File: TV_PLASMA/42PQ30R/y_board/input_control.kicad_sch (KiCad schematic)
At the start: 1 part, among them P101 Conn_02x15_Counter_Clockwise

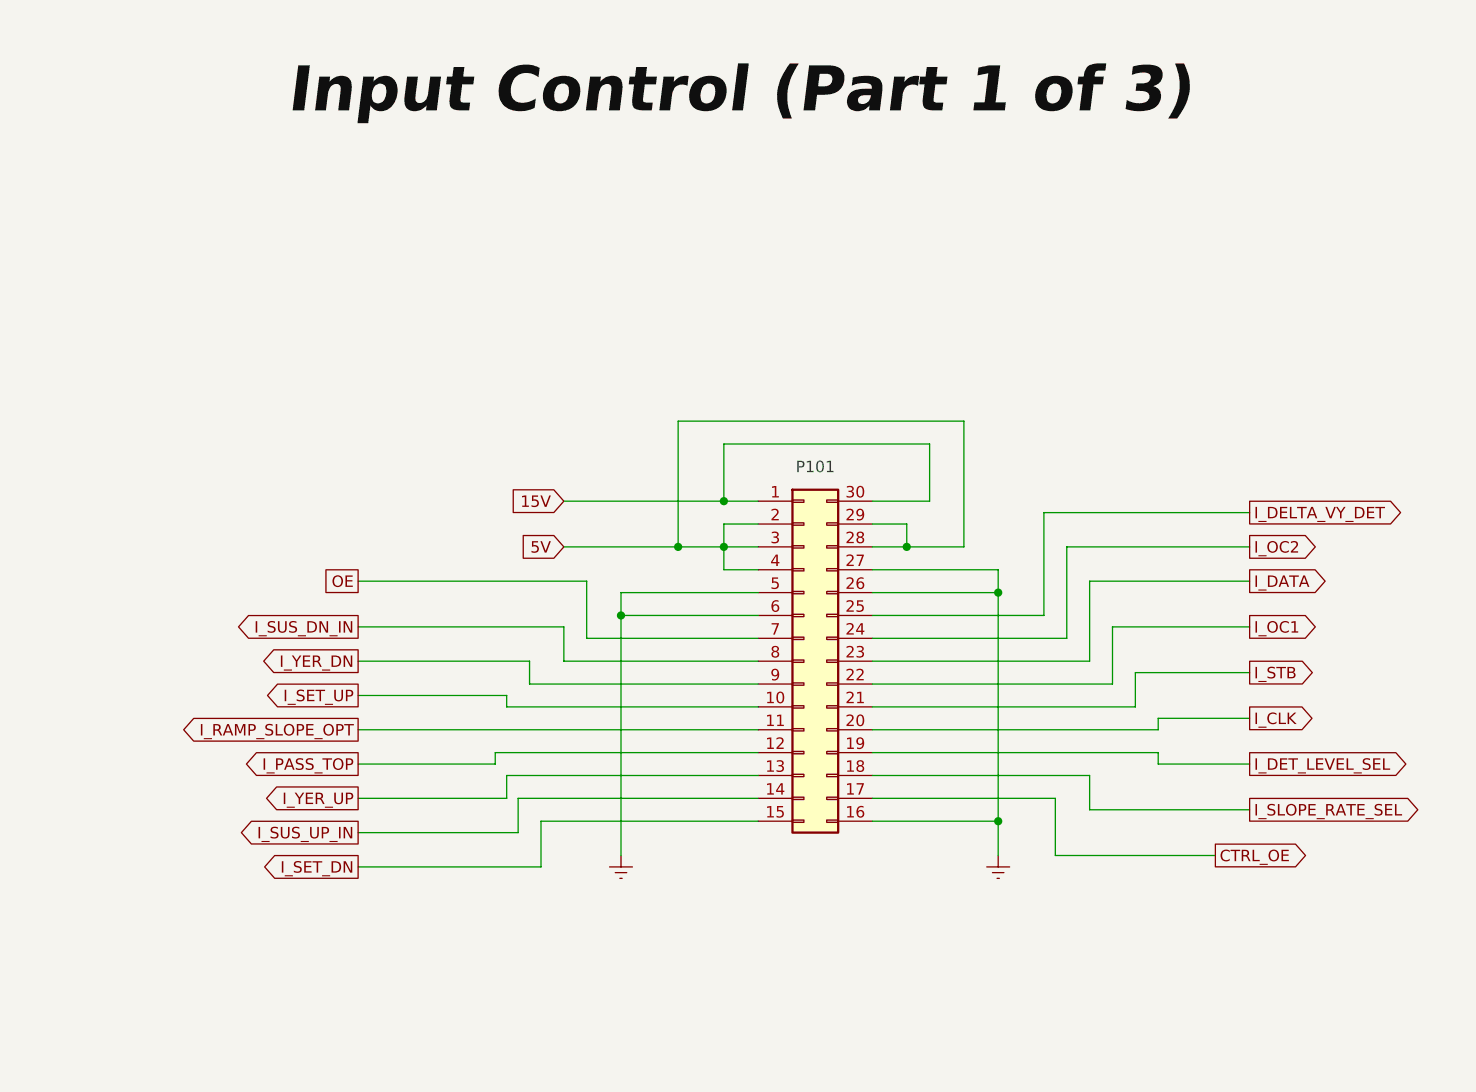
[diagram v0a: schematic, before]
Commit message: Finishing Y BOARD reverse engineering. Todo: Add reverse conduction and resistence to all output/input pins and refactor Z BOARD DRC
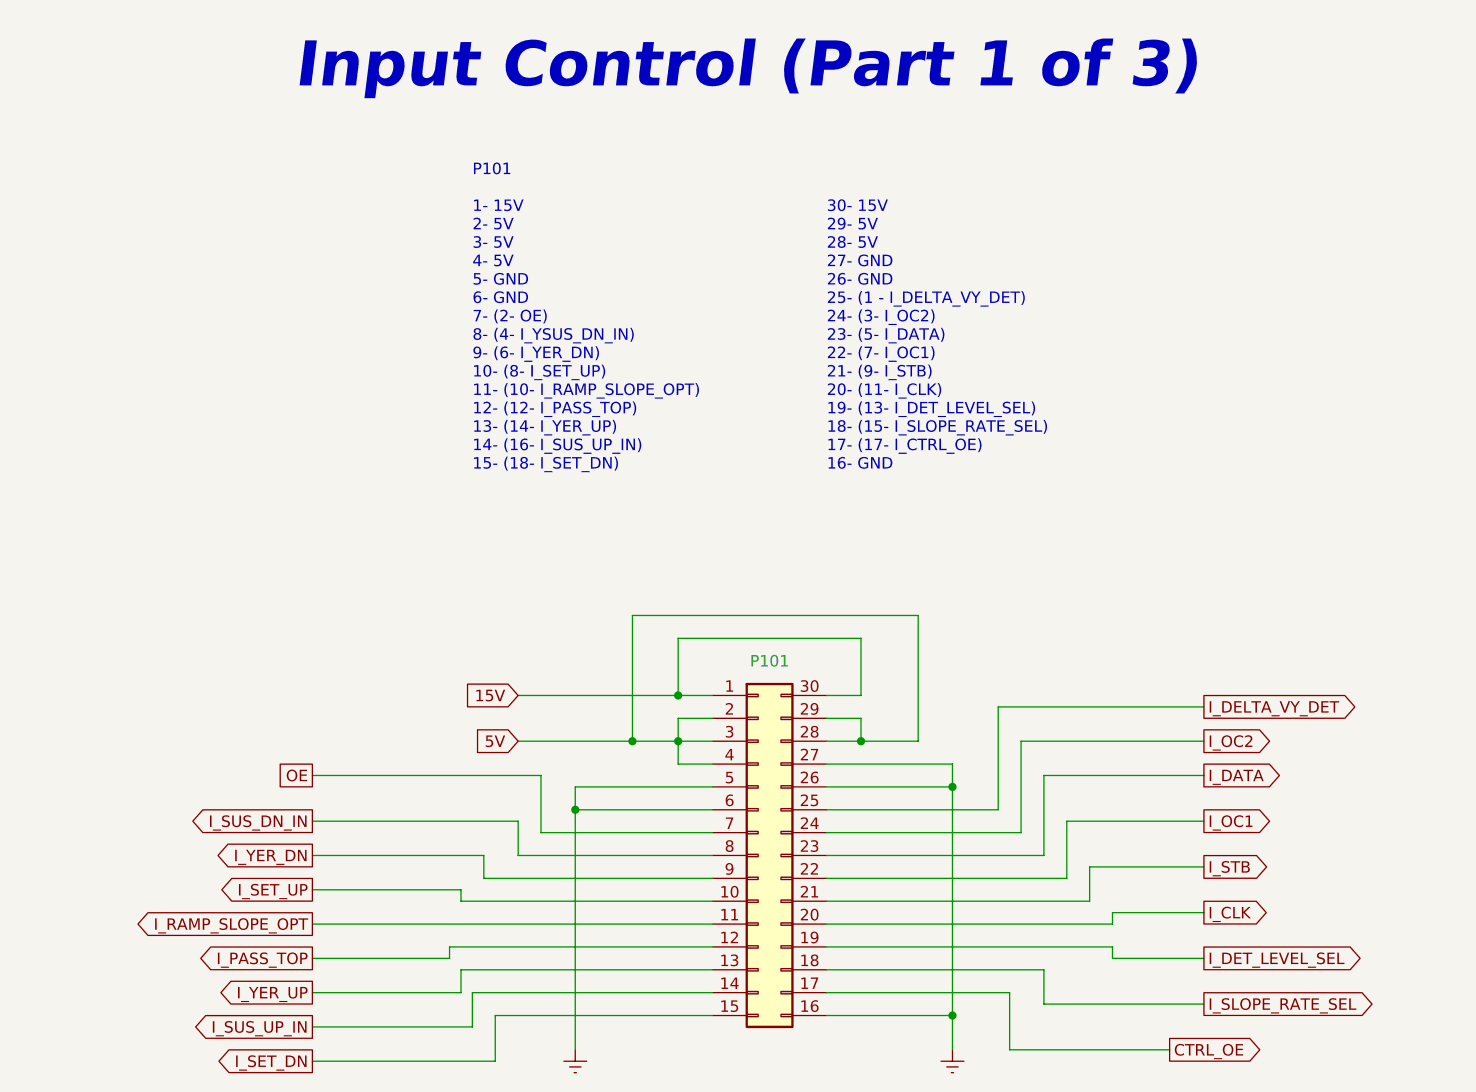
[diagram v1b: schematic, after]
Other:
- note added: "30- 15V 29- 5V 28- 5V 27- GND 26- GND 25- (1 - I_DELTA_VY_DET) 24- (3- I_OC2) 23- (5- I_DATA) 22- (7- I_OC1) 21- (9- I_STB) 20- (11- I_CLK) 19- (13- I_DET_LEVEL_SEL) 18- (15- I_SLOPE_RATE_SEL) 17- (17- I_CTRL_OE) 16- GND"
- note added: "Input Control (Part 1 of 3)"
- note added: "P101 1- 15V 2- 5V 3- 5V 4- 5V 5- GND 6- GND 7- (2- OE) 8- (4- I_YSUS_DN_IN) 9- (6- I_YER_DN) 10- (8- I_SET_UP) 11- (10- I_RAMP_SLOPE_OPT) 12- (12- I_PASS_TOP) 13- (14- I_YER_UP) 14- (16- I_SUS_UP_IN) 15- (18- I_SET_DN)"
- moved on the sheet: P101
